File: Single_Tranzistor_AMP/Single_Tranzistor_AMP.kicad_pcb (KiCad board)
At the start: 2 copper layers, 0 parts

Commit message: 6 nodarbibas majasdarbs
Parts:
- added BZ1: Buzzer, Buzzer_Beeper:Buzzer_D14mm_H7mm_P10mm, F.Cu at (98.4, 61.1)
- added C1: 10uF, Resistor_SMD:R_0805_2012Metric_Pad1.15x1.40mm_HandSolder, F.Cu at (117.1, 52.1)
- added C2: 10uF, Resistor_SMD:R_0805_2012Metric_Pad1.15x1.40mm_HandSolder, F.Cu at (108.0, 53.7)
- added C3: 10uF, Resistor_SMD:R_0805_2012Metric_Pad1.15x1.40mm_HandSolder, F.Cu at (106.5, 61.1)
- added J1: Screw_Terminal_01x03, TerminalBlock_4Ucon:TerminalBlock_4Ucon_1x03_P3.50mm_Vertical, F.Cu at (124.8, 52.6)
- added Q1: BC547, Package_TO_SOT_THT:TO-92_Inline, F.Cu at (114.2, 51.6)
- added Q2: BC557, Package_TO_SOT_THT:TO-92_Inline, F.Cu at (111.7, 60.6)
- added R1: 22K, Resistor_SMD:R_0805_2012Metric_Pad1.15x1.40mm_HandSolder, F.Cu at (117.2, 60.6)
- added R2: 6.8K, Resistor_SMD:R_0805_2012Metric_Pad1.15x1.40mm_HandSolder, F.Cu at (108.0, 56.1)
- added R3: 1K, Resistor_SMD:R_0805_2012Metric_Pad1.15x1.40mm_HandSolder, F.Cu at (113.1, 56.2)
- added R4: 560, Resistor_SMD:R_0805_2012Metric_Pad1.15x1.40mm_HandSolder, F.Cu at (106.7, 51.1)
- added R5: 1K, Resistor_SMD:R_0805_2012Metric_Pad1.15x1.40mm_HandSolder, F.Cu at (108.0, 58.7)
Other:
- board outline added: 40.2 x 17 mm

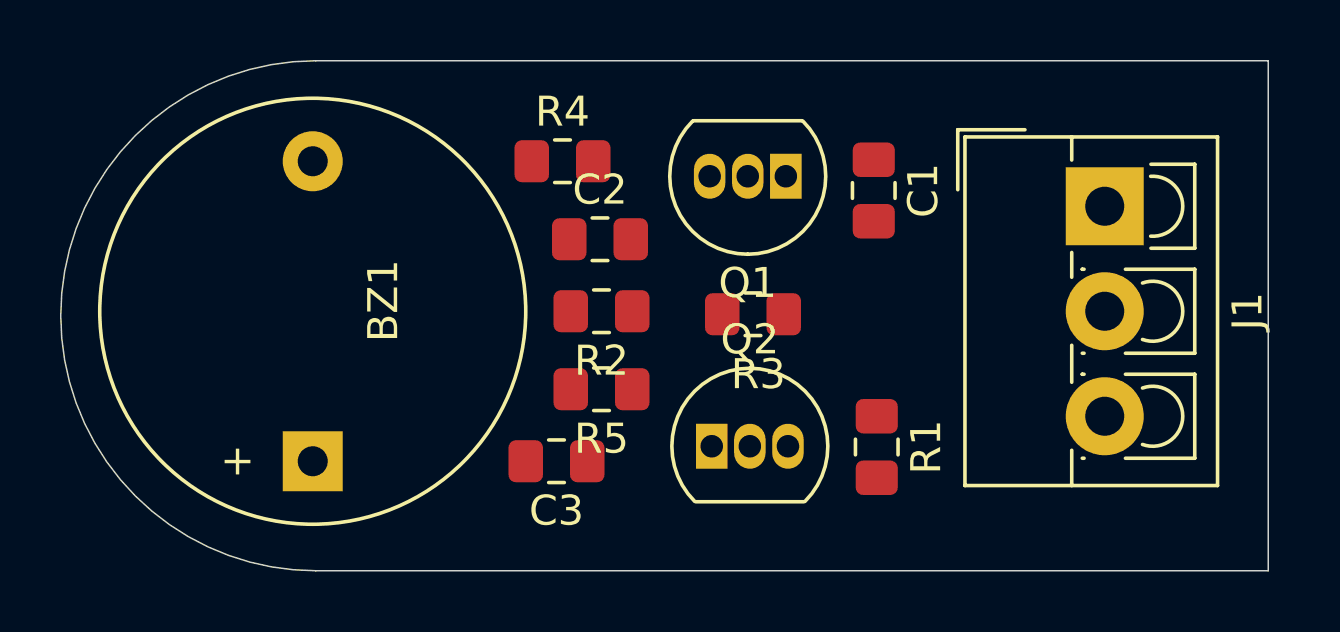
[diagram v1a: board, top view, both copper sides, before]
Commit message: majasdarbs par celinu trasesanu
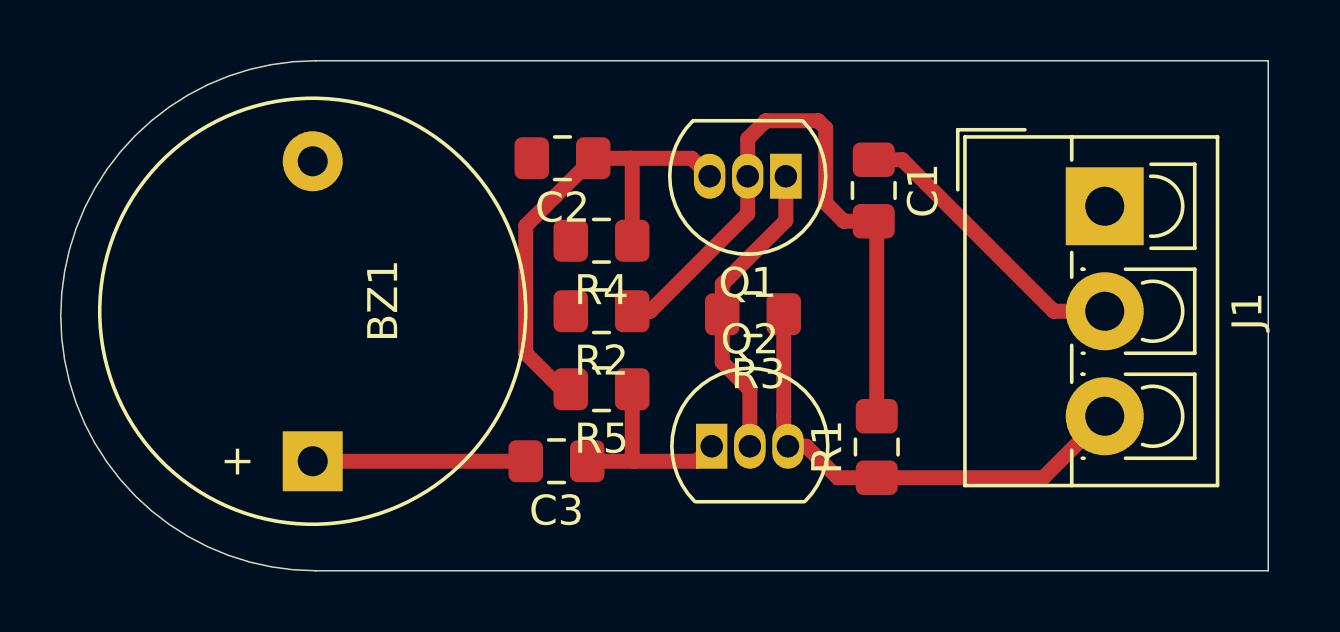
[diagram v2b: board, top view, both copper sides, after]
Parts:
- moved C2 2.98 mm to (106.7, 51.0), turned to 180 degrees
- moved R4 2.95 mm to (108.0, 53.8), turned to 180 degrees
- turned R1 to 90 degrees
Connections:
- net Net-(BZ1-Pad2) renamed GNDREF
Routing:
- net Net-(C1-Pad2): track 0.00 -> 21.5 mm
- net Net-(C2-Pad1): track 0.00 -> 16.3 mm
- net Net-(J1-Pad3): track 0.00 -> 16.3 mm
- net Net-(Q1-Pad1): track 0.00 -> 10.3 mm
- net Net-(C1-Pad1): track 0.00 -> 9.79 mm
- net Net-(BZ1-Pad1): track 0.00 -> 7.10 mm
- net Net-(C3-Pad1): track 0.00 -> 6.78 mm
